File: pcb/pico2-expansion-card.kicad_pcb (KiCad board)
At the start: 2 copper layers, 26 x 30.9 mm, 50 parts, among them J3 Conn_01x03_Socket, J4 Conn_01x04_Socket, Q1 EM6K6, Q2 EM6K6, SW1 SW_Push, U2 RP2354A, U4 AP2127K-3.3, Y1 ABM8-272-T3

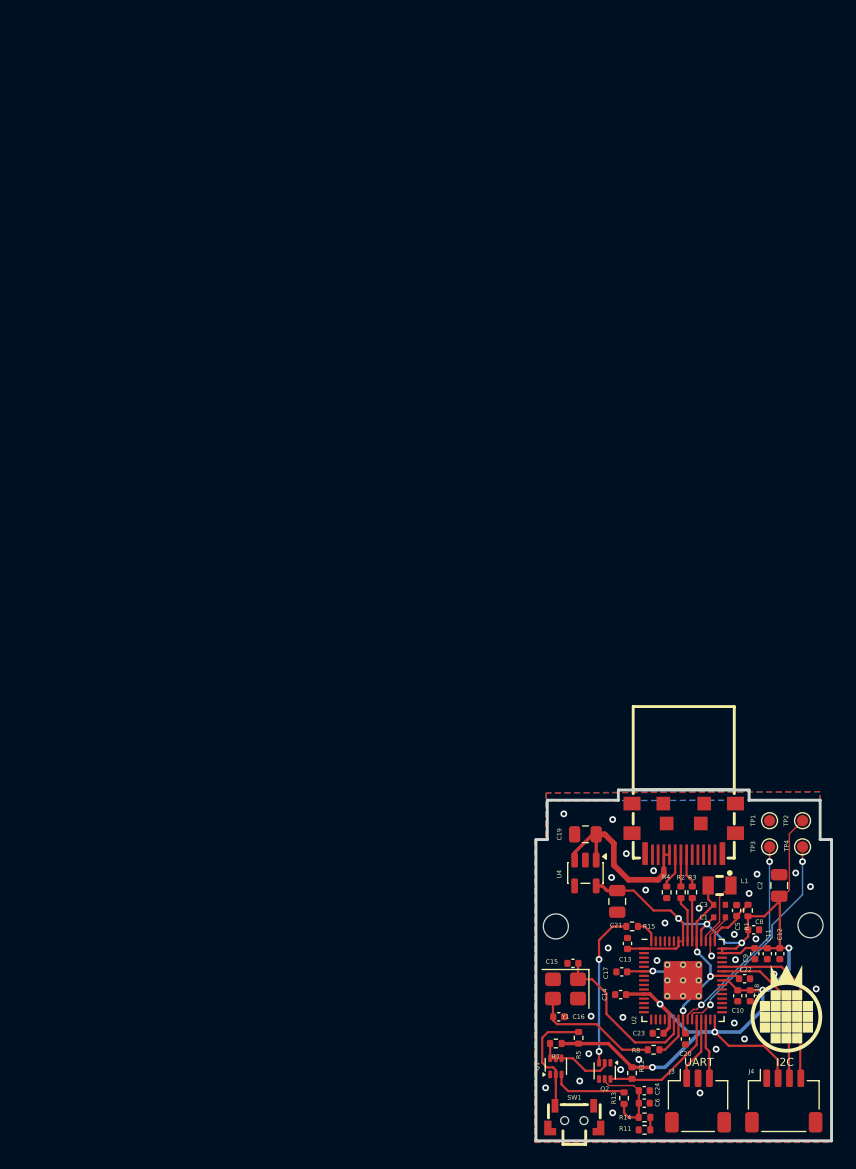
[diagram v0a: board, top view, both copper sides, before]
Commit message: cosmetic minor changes
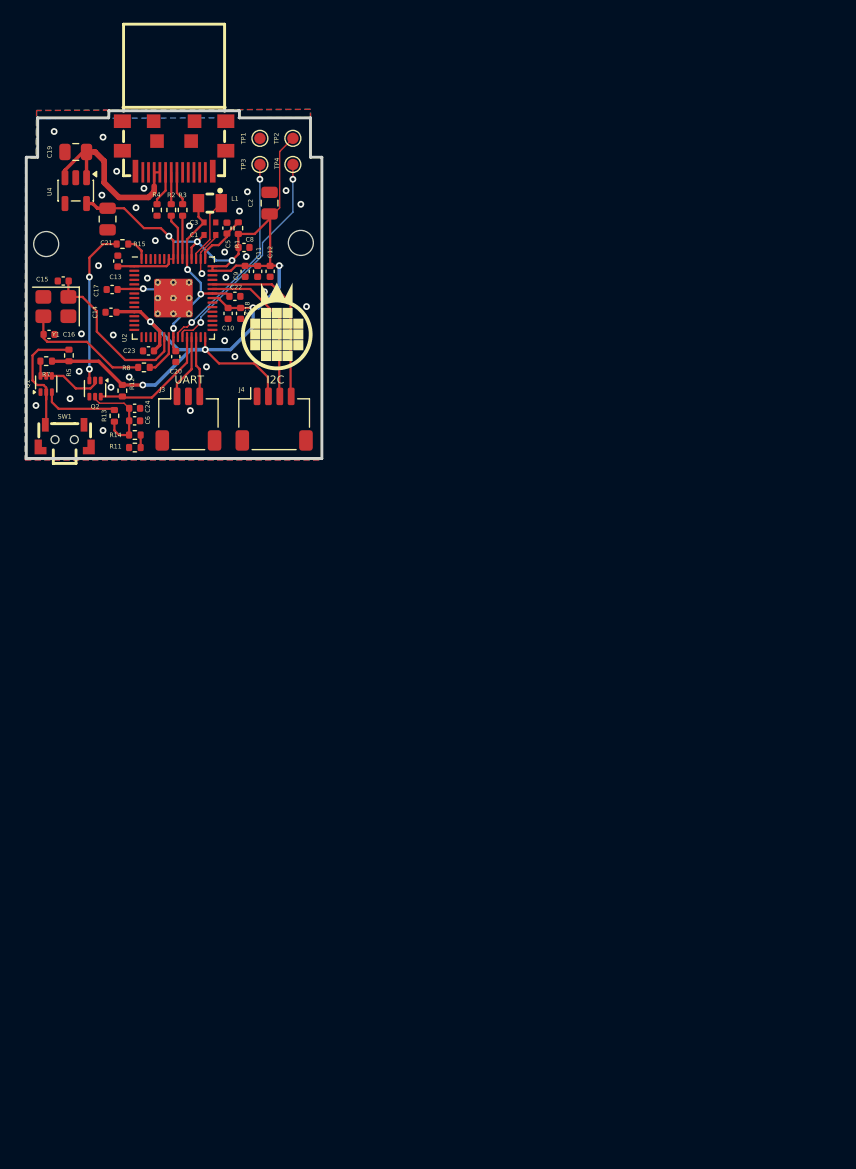
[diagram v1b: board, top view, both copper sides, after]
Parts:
- moved C10 74.9 mm to (109.7, 75.2)
- moved C11 74.9 mm to (112.3, 71.5)
- moved C15 74.9 mm to (95.2, 72.4)
- moved C16 74.9 mm to (93.9, 77.1)
- moved C18 74.9 mm to (110.8, 75.2)
- moved C22 74.9 mm to (110.3, 73.7)
- moved C23 74.9 mm to (102.7, 78.5)
- moved C24 74.9 mm to (101.5, 83.6)
- moved C6 74.9 mm to (101.5, 84.7)
- moved C9 74.9 mm to (111.2, 71.5)
- moved H1 74.9 mm to (93.7, 69.1)
- moved Q1 74.9 mm to (93.7, 81.4)
- moved R13 74.9 mm to (99.7, 84.2)
- moved R2 74.9 mm to (104.7, 66.1)
- moved R3 74.9 mm to (105.7, 66.1)
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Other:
- board size 26 x 30.9 mm -> 26 x 30.6 mm

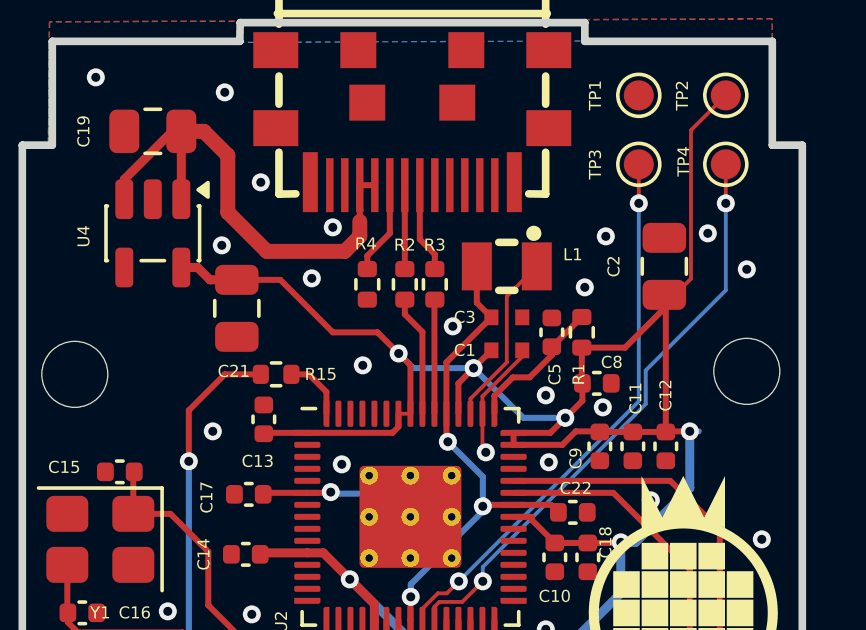
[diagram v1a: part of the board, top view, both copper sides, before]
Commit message: fix connections
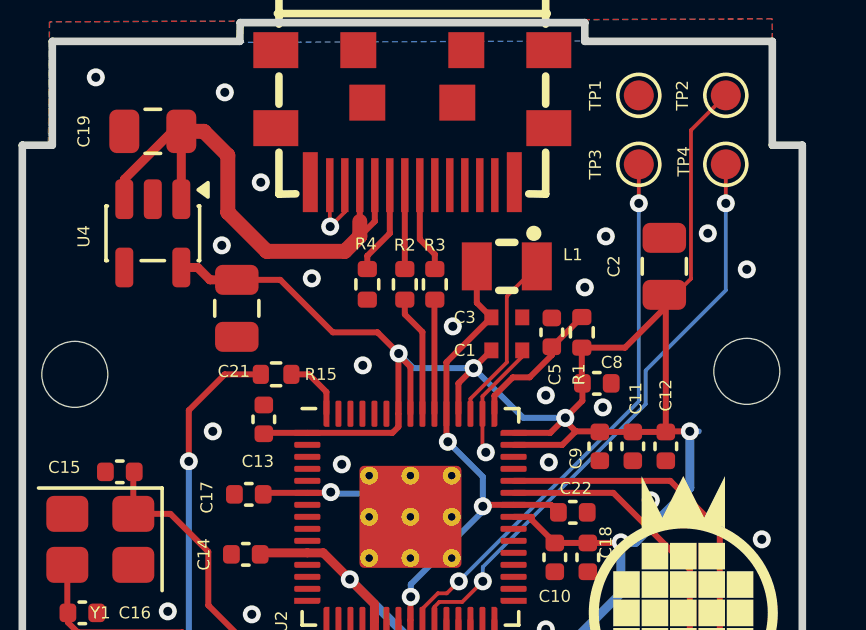
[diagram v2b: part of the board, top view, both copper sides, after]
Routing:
- net GND: track 4.04 -> 7.01 mm
- net +3.3V: track 105.1 -> 106.9 mm
- net VBUS: track 16.6 -> 18.0 mm
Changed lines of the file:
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@@
+	)
+	(segment
+		(start 102.2 64.2)
+		(end 102.18745 64.18745)
+		(width 0.127)
+		(layer "F.Cu")
+		(net "GND")
+	)
+	(segment
+		(start 102.18745 64.18745)
+		(end 102.18745 62.8185)
+		(width 0.127)
+		(layer "F.Cu")
+		(net "GND")
+	)
+	(segment
+		(start 102.68755 63.71245)
+		(end 102.2 64.2)
+		(width 0.127)
+		(layer "F.Cu")
+		(net "GND")
 	)
 	(segment
@@
 	)
 	(segment
+		(start 102.68755 62.8185)
+		(end 102.68755 63.71245)
+		(width 0.127)
+		(layer "F.Cu")
+		(net "GND")
+	)
+	(segment
 		(start 107.275 70.4375)
 		(end 107.275 69.858526)
@@
 	)
 	(via
-		(at 102.2875 64.225)
+		(at 102.2 64.2)
 		(size 0.6)
 		(drill 0.3)
@@
 	)
 	(segment
+		(start 110.00625 70.64375)
+		(end 110.3875 71.025)
+		(width 0.2)
+		(layer "F.Cu")
+		(net "+3.3V")
+	)
+	(segment
 		(start 108.9175 73.975)
 		(end 109.6875 74.745)
@@
 	)
 	(segment
-		(start 104.482977 68.429523)
-		(end 104.875 68.821545)
-		(width 0.2)
-		(layer "F.Cu")
-		(net "+3.3V")
-	)
-	(segment
 		(start 94.2075 79.435)
 		(end 94.1975 79.425)
@@
 	)
 	(segment
-		(start 104.875 70.4375)
-		(end 104.475 70.4375)
-		(width 0.127)
-		(layer "F.Cu")
-		(net "+3.3V")
-	)
-	(segment
 		(start 108.9175 73.875)
 		(end 108.9175 73.975)
@@
 	)
 	(segment
-		(start 104.875 68.821545)
-		(end 104.875 70.4375)
+		(start 104.875 70.4375)
+		(end 104.875 68.875)
 		(width 0.2)
 		(layer "F.Cu")
@@
 	)
 	(segment
+		(start 110.00625 70.60625)
+		(end 110.00625 70.64375)
+		(width 0.2)
+		(layer "F.Cu")
+		(net "+3.3V")
+	)
+	(segment
+		(start 104.482977 68.482977)
+		(end 104.482977 68.429523)
+		(width 0.2)
+		(layer "F.Cu")
+		(net "+3.3V")
+	)
+	(segment
 		(start 98.3075 79.435)
 		(end 100.3875 81.515)
@@
 	)
 	(segment
+		(start 110.0375 70.575)
+		(end 110.00625 70.60625)
+		(width 0.2)
+		(layer "F.Cu")
+		(net "+3.3V")
+	)
+	(segment
 		(start 103.675 78.0175)
 		(end 103.675 77.3125)
@@
 	)
 	(segment
+		(start 104.475 68.4375)
+		(end 104.482977 68.429523)
+		(width 0.2)
+		(layer "F.Cu")
+		(net "+3.3V")
+	)
+	(segment
 		(start 98.19375 65.975)
 		(end 97.78125 65.5625)
@@
 	)
 	(segment
+		(start 104.475 70.4375)
+		(end 104.475 68.4375)
+		(width 0.2)
+		(layer "F.Cu")
+		(net "+3.3V")
+	)
+	(segment
+		(start 104.875 68.875)
+		(end 104.482977 68.482977)
+		(width 0.2)
+		(layer "F.Cu")
+		(net "+3.3V")
+	)
+	(segment
 		(start 108.3125 73.875)
 		(end 108.9175 73.875)
@@
 		(start 107.5725 68.325)
 		(end 106.98 68.9175)
-		(width 0.2)
-		(layer "F.Cu")
-		(net "+3.3V")
-	)
-	(segment
-		(start 108.3125 71.475)
-		(end 108.3125 71.075)
 		(width 0.2)
 		(layer "F.Cu")
@@
 	)
 	(segment
+		(start 103.68755 62.8185)
+		(end 103.68755 64.02495)
+		(width 0.2)
+		(layer "F.Cu")
+		(net "VBUS")
+	)
+	(segment
+		(start 103.68755 64.02495)
+		(end 103.1875 64.525)
+		(width 0.2)
+		(layer "F.Cu")
+		(net "VBUS")
+	)
+	(segment
 		(start 96.937501 61.025)
 		(end 95.3375 62.625001)
@@
 		(end 96.937501 61.025)
 		(width 0.3)
-		(layer "F.Cu")
-		(net "VBUS")
-	)
-	(segment
-		(start 103.68755 62.8185)
-		(end 103.18745 62.8185)
-		(width 0.2)
 		(layer "F.Cu")
 		(net "VBUS")
@@
 	)
 	(zone
+		(layer "F.Cu")
+		(hatch edge 0.5)
+		(connect_pads
+			(clearance 0)
+		)
+		(min_thickness 0.25)
+		(keepout
+			(tracks not_allowed)
+			(vias not_allowed)
+			(pads not_allowed)
+			(copperpour not_allowed)
+			(footprints allowed)
+		)
+		(placement
+			(enabled no)
+			(sheetname "")
+		)
+		(fill
+			(thermal_gap 0.5)
+			(thermal_bridge_width 0.5)
+			(island_removal_mode 0)
+		)
+		(polygon
+			(pts
+				(xy 100.4 57.4) (xy 109.4 57.4) (xy 109.4 63.2) (xy 100.4 63.2)
+			)
+		)
+	)
+	(zone
